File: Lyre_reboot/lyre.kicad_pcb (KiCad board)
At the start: 2 copper layers, 78.2 x 68.8 mm, 1 part

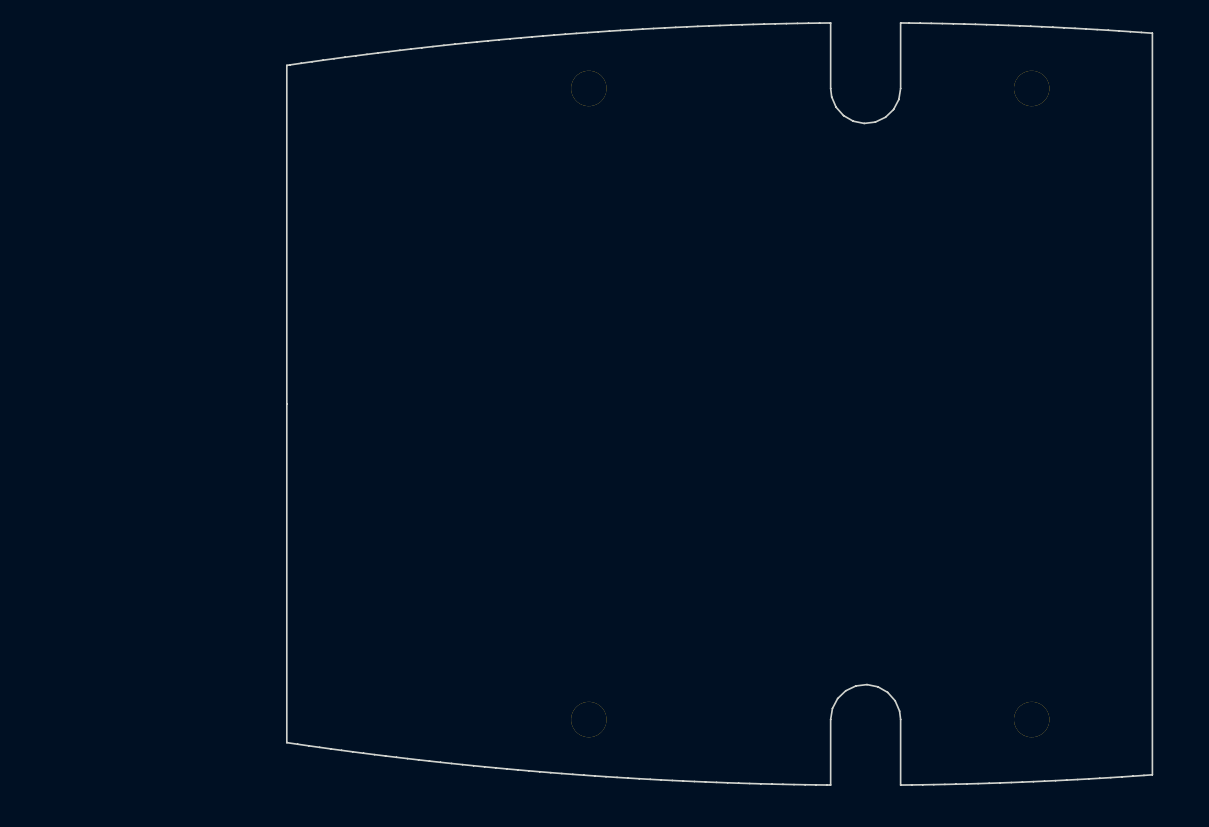
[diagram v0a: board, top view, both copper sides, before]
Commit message: Lyre_reboot: Update
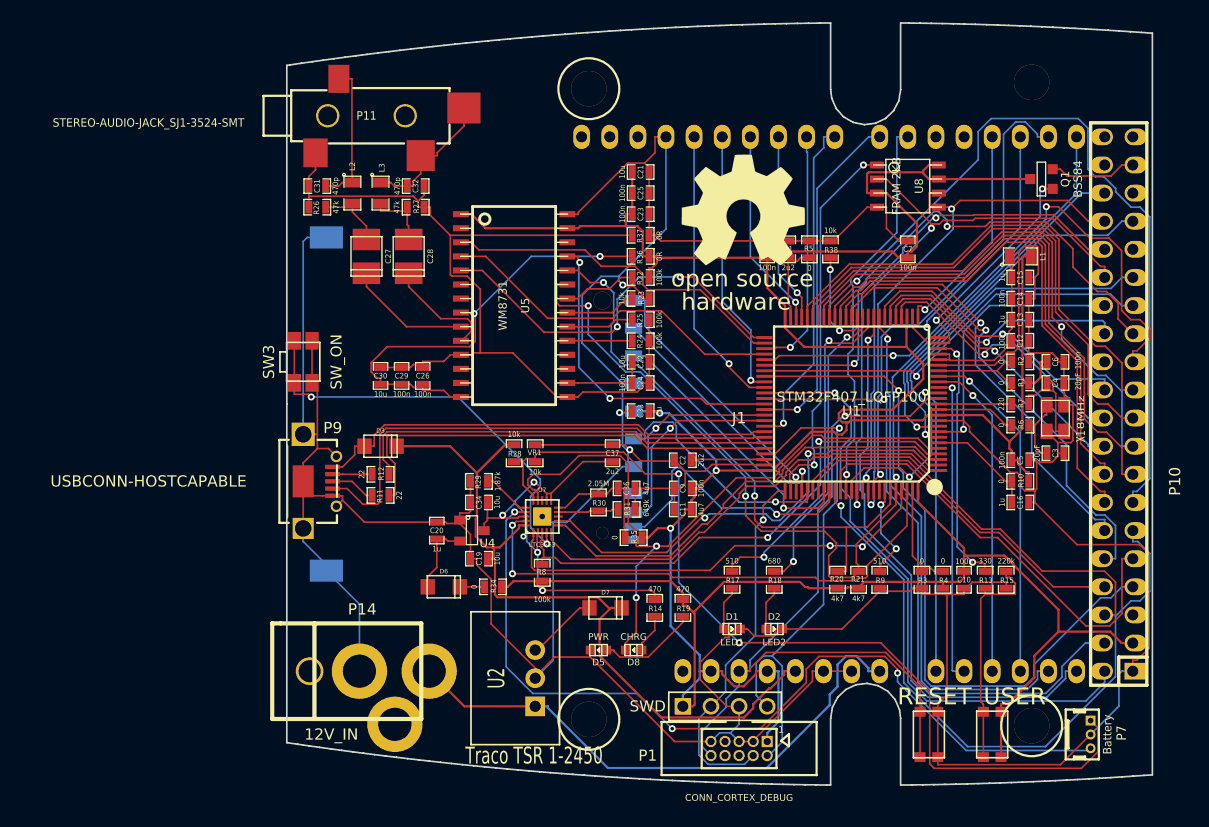
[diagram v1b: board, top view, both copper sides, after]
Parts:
- removed pcb_hammond_1553bbat: VAL**, pcb_hammond_1553bbat
- added C1: 2u2, SM0603_Capa, F.Cu at (121.3, 113.0)
- added C10: 100n, SM0603_Capa, F.Cu at (137.2, 142.9)
- added C11: 4u7, SM0603_Capa, F.Cu at (111.8, 136.5)
- added C12: 100n, SM0603_Capa, F.Cu at (142.2, 121.3)
- added C13: 1u, SM0603_Capa, F.Cu at (142.2, 119.4)
- added C14: 100n, SM0603_Capa, F.Cu at (142.2, 117.5)
- added C15: 1u, SM0603_Capa, F.Cu at (142.2, 115.6)
- added C16: 1u, SM0603_Capa, F.Cu at (142.2, 135.9)
- added C19: 10u, SM0603_Capa, F.Cu at (93.3, 141.0)
- added C2: 2u2, SM0603_Capa, F.Cu at (111.8, 132.1)
- added C20: 1u, SM0603_Capa, F.Cu at (89.5, 138.4)
- added C21: 10u, SM0603_Capa, F.Cu at (108.0, 106.0)
- added C22: 10u, SM0603_Capa, F.Cu at (108.0, 123.2)
- added C23: 100n, SM0603_Capa, F.Cu at (108.0, 109.9)
- added C24: 100n, SM0603_Capa, F.Cu at (108.0, 125.1)
- added C25: 100n, SM0603_Capa, F.Cu at (108.0, 108.0)
- added C26: 100n, SM0603_Capa, F.Cu at (88.3, 124.5)
- added C27: 220u, c_tant_B, F.Cu at (83.2, 113.7)
- added C28: 220u, c_tant_B, F.Cu at (87.0, 113.7)
- added C29: 100n, SM0603_Capa, F.Cu at (86.4, 124.5)
- added C3: 20pF, SM0603_Capa, F.Cu at (145.4, 131.4)
- added C30: 10u, SM0603_Capa, F.Cu at (84.5, 124.5)
- added C31: 470p, SM0603_Capa, F.Cu at (78.7, 107.3)
- added C32: 470p, SM0603_Capa, F.Cu at (87.6, 107.3)
- added C33: 1u, SM0603_Capa, F.Cu at (108.0, 127.6)
- added C34: 10u, SM0603_Capa, F.Cu at (93.3, 135.9)
- added C36: 4u7, SM0603_Capa, F.Cu at (106.7, 134.6)
- added C37: 2u2, SM0603_Capa, F.Cu at (105.4, 131.4)
- added C4: 20pF, SM0603_Capa, F.Cu at (145.4, 125.1)
- added C5: 100n, SM0603_Capa, F.Cu at (142.2, 132.1)
- added C6: 100n, SM0603_Capa, F.Cu at (145.4, 123.2)
- added C7: 100n, SM0603_Capa, F.Cu at (132.1, 113.0)
- added C8: 100n, SM0603_Capa, F.Cu at (119.4, 113.0)
- added C9: 100n, SM0603_Capa, F.Cu at (111.8, 134.6)
- added D1: LED1, Led_0603, F.Cu at (116.2, 147.3)
- added D2: LED2, Led_0603, F.Cu at (120.0, 147.3)
- added D3: DIODE, do219ab, F.Cu at (84.5, 130.8)
- added D5: PWR, Led_0603, F.Cu at (104.1, 149.2)
- added D6: DIODE, do219ab, F.Cu at (90.2, 143.5)
- added D7: DIODE, do219ab, F.Cu at (104.8, 145.4)
- added D8: CHRG, Led_0603, F.Cu at (107.3, 149.2)
- added J1: ARDUINO_HEADER, arduino_header_bare, F.Cu at (116.8, 127.0)
- added L1: L_MINI, SM0805, F.Cu at (142.2, 113.7)
- added L2: INDUCTOR_SMALL, SM0805, F.Cu at (81.9, 108.0)
- added L3: INDUCTOR_SMALL, SM0805, F.Cu at (84.5, 108.0)
- added M1: LOGO_OSHW, OSHW_logo_2, F.Cu at (117.2, 109.5)
- added M2: Hammond_PCB, pcb_hammond_1553bbat, F.Cu at (128.3, 127.0)
- added P1: SWD, pin_header_2.54mm_1x4, F.Cu at (115.6, 154.3)
- added P10: LCD_2.4_INCH, pin_socket_20x2, F.Cu at (151.1, 127.0)
- added P11: STEREO-AUDIO-JACK_SJ1-3524-SMT, SJ-3524-SMT_Stereo_Jack, F.Cu at (83.2, 101.0)
- added P13: CONN_SD, Memory_Card_SD_3M, B.Cu at (107.3, 127.0)
- added P14: 12V_IN, JACK_PWR, F.Cu at (82.5, 151.1)
- added P7: Battery, BATTery_Molex_53047-0310, F.Cu at (148.6, 156.8)
- added P8: CONN_CORTEX_DEBUG, Pin_Array_5x2_1.27mm_RMC, F.Cu at (116.8, 158.1)
- added P9: USBCONN-HOSTCAPABLE, USB_MICRO_RMC, F.Cu at (77.5, 134.0)
- added Q1: BSS84, SOT23GDS, F.Cu at (144.1, 106.7)
- added R1: 0, SM0603_Resistor, F.Cu at (142.2, 125.1)
- added R10: 0, SM0603_Resistor, F.Cu at (142.2, 134.0)
- added R11: 22, SM0603_Resistor, F.Cu at (84.5, 135.3)
- added R12: 22, SM0603_Resistor, F.Cu at (84.5, 133.3)
- added R13: 330, SM0603_Resistor, F.Cu at (139.1, 142.9)
- added R14: 470, SM0603_Resistor, F.Cu at (109.2, 145.4)
- added R15: 220k, SM0603_Resistor, F.Cu at (141.0, 142.9)
- added R17: 510, SM0603_Resistor, F.Cu at (116.2, 142.9)
- added R18: 680, SM0603_Resistor, F.Cu at (120.0, 142.9)
- added R19: 470, SM0603_Resistor, F.Cu at (111.8, 145.4)
- added R2: 0, SM0603_Resistor, F.Cu at (142.2, 123.2)
- added R20: 4k7, SM0603_Resistor, F.Cu at (125.7, 142.9)
- added R21: 4k7, SM0603_Resistor, F.Cu at (127.6, 142.9)
- added R22: 100k, SM0603_Resistor, F.Cu at (108.0, 115.6)
- added R23: 10k, SM0603_Resistor, F.Cu at (108.0, 117.5)
- added R24: 100k, SM0603_Resistor, F.Cu at (108.0, 121.3)
- added R25: 100k, SM0603_Resistor, F.Cu at (108.0, 119.4)
- added R26: 47k, SM0603_Resistor, F.Cu at (78.7, 109.2)
- added R27: 47k, SM0603_Resistor, F.Cu at (87.6, 109.2)
- added R28: 10k, SM0603_Resistor, F.Cu at (96.5, 131.4)
- added R29: 1.87k, SM0603_Resistor, F.Cu at (93.3, 134.0)
- added R3: 0, SM0603_Resistor, F.Cu at (133.3, 142.9)
- added R30: 2.05M, SM0603_Resistor, F.Cu at (104.1, 135.9)
- added R31: 649k, SM0603_Resistor, F.Cu at (106.7, 136.5)
- added R34: 0, SM0603_Resistor, F.Cu at (94.6, 143.5)
- added R35: 0, SM0603_Resistor, F.Cu at (107.3, 139.1)
- added R36: 0R, SM0603_Resistor, F.Cu at (108.0, 113.7)
- added R37: 0R, SM0603_Resistor, F.Cu at (108.0, 111.8)
- added R38: 10k, SM0603_Resistor, F.Cu at (125.1, 113.0)
- added R4: 0, SM0603_Resistor, F.Cu at (135.3, 142.9)
- added R5: 0, SM0603_Resistor, F.Cu at (123.2, 113.0)
- added R6: 0, SM0603_Resistor, F.Cu at (142.2, 128.9)
- added R7: 220, SM0603_Resistor, F.Cu at (142.2, 127.0)
- added R8: 100k, SM0603_Resistor, F.Cu at (99.1, 142.2)
- added R9: 510, SM0603_Resistor, F.Cu at (129.5, 142.9)
- added SW1: USER, SW_C&K_KMR4, F.Cu at (139.7, 156.8)
- added SW2: RESET, SW_C&K_KMR4, F.Cu at (134.0, 156.8)
- added SW3: SW_ON, sw_panasonic_evqp7, F.Cu at (77.5, 123.2)
- added U1: STM32F407_LQFP100, LQFP100_0.5mm_SOT407-1_LPC1768, F.Cu at (127.0, 127.0)
- added U2: Traco TSR 1-2450, Traco_TSR-1, F.Cu at (98.4, 151.8)
- added U4: MCP1703_SOT23, SOT23, F.Cu at (92.7, 138.4)
- added U5: WM8731, soic-28, F.Cu at (96.5, 118.1)
- added U7: LTC3553, qfn-20-LTC3553, F.Cu at (99.1, 137.2)
- added U8: FRAM 2KB, so-8, F.Cu at (132.1, 107.3)
- added VR1: 10k, SM0603_Resistor, F.Cu at (98.4, 131.4)
- added X1: 8MHz, XTAL-3.2x2.5mm, F.Cu at (145.4, 128.3)
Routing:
- net GND: track 0.00 -> 452.8 mm, vias 0 -> 3
- net VDD: track 0.00 -> 325.8 mm, vias 0 -> 3
- net AGND_AUDIO: track 0.00 -> 84.0 mm
- net /Power/BAT_THERMISTOR: track 0.00 -> 82.6 mm, vias 0 -> 2
- net /Power/V_BAT: track 0.00 -> 78.2 mm, vias 0 -> 3
- net D8: track 0.00 -> 71.1 mm, vias 0 -> 1
- net NRST: track 0.00 -> 71.0 mm, vias 0 -> 1
- net +5V: track 0.00 -> 68.0 mm
- net LCD_RS: track 0.00 -> 63.2 mm, vias 0 -> 1
- net nCHRG: track 0.00 -> 63.1 mm, vias 0 -> 2
- net LCD_RD: track 0.00 -> 60.0 mm, vias 0 -> 1
- net D1: track 0.00 -> 57.4 mm, vias 0 -> 1
- net D0: track 0.00 -> 56.2 mm, vias 0 -> 1
- net AUDIO_SDA: track 0.00 -> 55.4 mm, vias 0 -> 2
- net D13: track 0.00 -> 52.7 mm, vias 0 -> 2
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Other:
- outline, holes or cut-outs redrawn
- net class Default: clearance 0.254 -> 0.1524; trace_width 0.254 -> 0.1524; via_dia 0.889 -> 0.635; via_drill 0.635 -> 0.3302
- net class power added: clearance 0.1524, trace_width 0.2032, via_dia 0.635, via_drill 0.3302
- rule trace_clearance: 0.254 -> 0.1524
- rule trace_min: 0.254 -> 0.1524
- rule via_min_drill: 0.508 -> 0.3302
- rule via_min_size: 0.889 -> 0.635
